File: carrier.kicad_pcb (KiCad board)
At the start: 4 copper layers, 20.3 x 68.6 mm, 30 parts, among them J1 Conn_02x06_Odd_Even, J2 Conn_01x26, J3 Conn_01x26, U1 CARAVEL, U2 W25Q128JVS, U3 LP5907MFX-3.3, U4 LP5907MFX-1.8, U5 LP5907MFX-1.8, U6 LP5907MFX-3.3, X1 SG-5032CAN

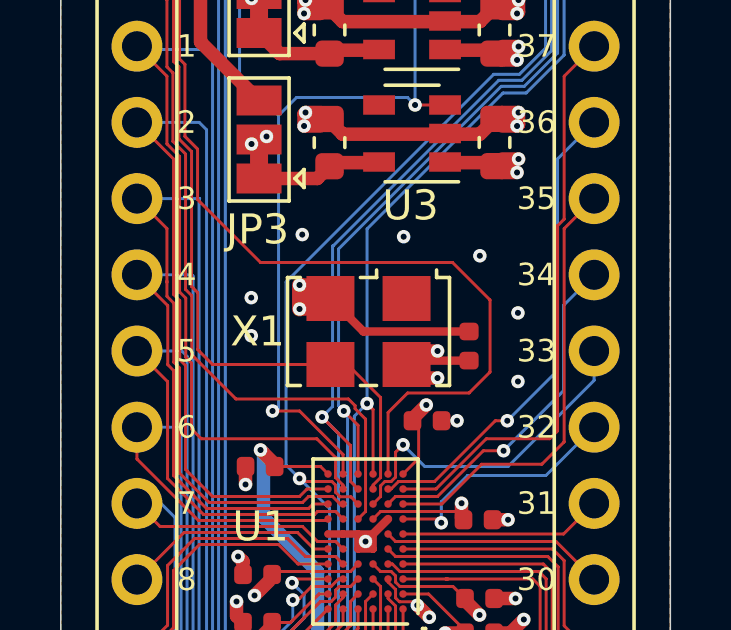
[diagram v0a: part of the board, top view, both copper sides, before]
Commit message: Tidy up oscillator.
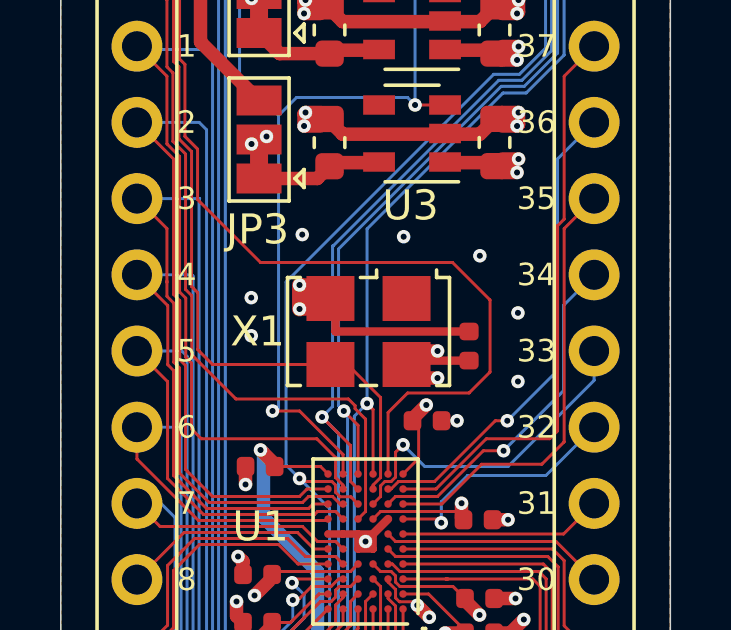
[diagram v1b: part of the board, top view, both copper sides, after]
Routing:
- net GND: track 61.7 -> 62.2 mm
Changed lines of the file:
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@@
     (thickness 1.6)
     (drawings 75)
-    (tracks 1055)
+    (tracks 1056)
     (zones 0)
     (modules 30)
@@
     (effects (font (size 0.75 0.75) (thickness 0.1)) (justify left))
   )
-  (gr_poly (pts (xy 66.93 72.8) (xy 71.33 72.8) (xy 71.33 73.2) (xy 66.93 73.2)) (layer F.Mask) (width 0.1))
+  (gr_poly (pts (xy 67.48 72.8) (xy 71.33 72.8) (xy 71.33 73.2) (xy 67.48 73.2)) (layer F.Mask) (width 0.1))
   (gr_line (start 78.89 43.17) (end 78.89 111.75) (layer Edge.Cuts) (width 0.05))
   (gr_line (start 58.57 43.17) (end 78.89 43.17) (layer Edge.Cuts) (width 0.05))
@@
   (segment (start 66.68 65.75) (end 66.73 65.7) (width 0.45) (layer F.Cu) (net 3))
   (segment (start 66.68 66.15) (end 66.68 65.75) (width 0.45) (layer F.Cu) (net 3))
-  (segment (start 68.6584 73) (end 67.5584 71.9) (width 0.28) (layer F.Cu) (net 3) (status 20))
-  (segment (start 72.18 73) (end 68.6584 73) (width 0.28) (layer F.Cu) (net 3) (status 10))
   (via (at 66.53 71.45) (size 0.45) (drill 0.2) (layers F.Cu B.Cu) (net 3))
   (via (at 66.53 72.25) (size 0.45) (drill 0.2) (layers F.Cu B.Cu) (net 3))
@@
   (segment (start 69.859999 82.009999) (end 69.73 81.88) (width 0.1) (layer F.Cu) (net 3))
   (segment (start 70.455 82.125) (end 70.339999 82.009999) (width 0.1) (layer F.Cu) (net 3))
+  (segment (start 67.73 72.0716) (end 67.5584 71.9) (width 0.28) (layer F.Cu) (net 3))
+  (segment (start 67.73 73) (end 67.73 72.0716) (width 0.28) (layer F.Cu) (net 3))
+  (segment (start 72.18 73) (end 67.73 73) (width 0.28) (layer F.Cu) (net 3))
   (via (at 74.064 103.622) (size 0.45) (drill 0.2) (layers F.Cu B.Cu) (net 4))
   (via (at 73.556 103.622) (size 0.45) (drill 0.2) (layers F.Cu B.Cu) (net 4))
@@
       )
     )
+  )
+  (zone (net 0) (net_name "") (layer F.Cu) (hatch edge 0.508)
+    (connect_pads (clearance 0.2))
+    (min_thickness 0.254)
+    (keepout (tracks allowed) (vias allowed) (copperpour not_allowed))
+    (fill (arc_segments 32) (thermal_gap 0.508) (thermal_bridge_width 0.508))
+    (polygon
+      (pts
+        (xy 72.73 72) (xy 72.73 75) (xy 66.73 75) (xy 66.73 70.5) (xy 71.23 70.5)
+      )
+    )
